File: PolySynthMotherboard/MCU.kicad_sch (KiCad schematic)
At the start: 45 parts, among them J201 SWD Header, J202 USB_C_Leceptacle_USB2.0, J203 MIDI_In, J204 MIDI_Thru, J205 MIDI_Out, J401 Micro_SD_Card_Det2, SW201 RST, SW202 BOOT, U201 STM32F411RETx, U202 74HC595, U203 74HC595, U204 4N35, U205 74HC04, Y201 16MHz, Y202 32.768kHZ

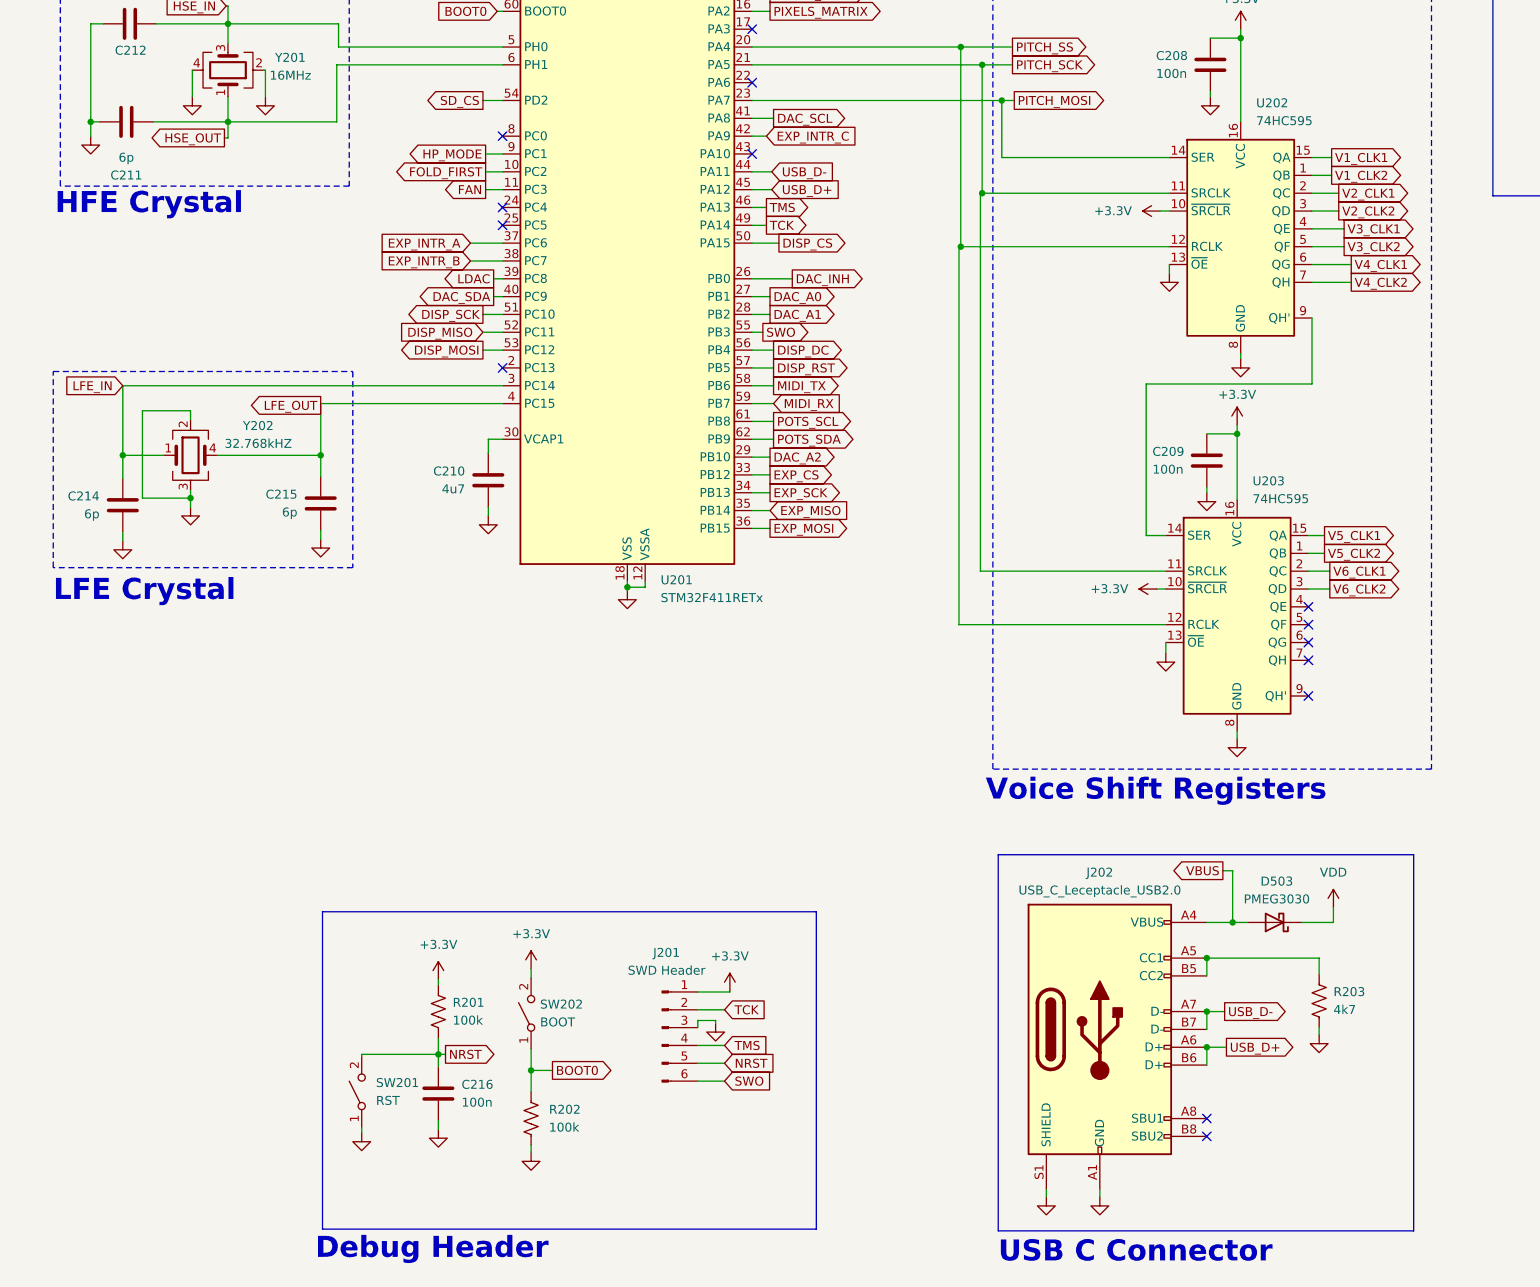
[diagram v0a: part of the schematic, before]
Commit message: motherboard rev1
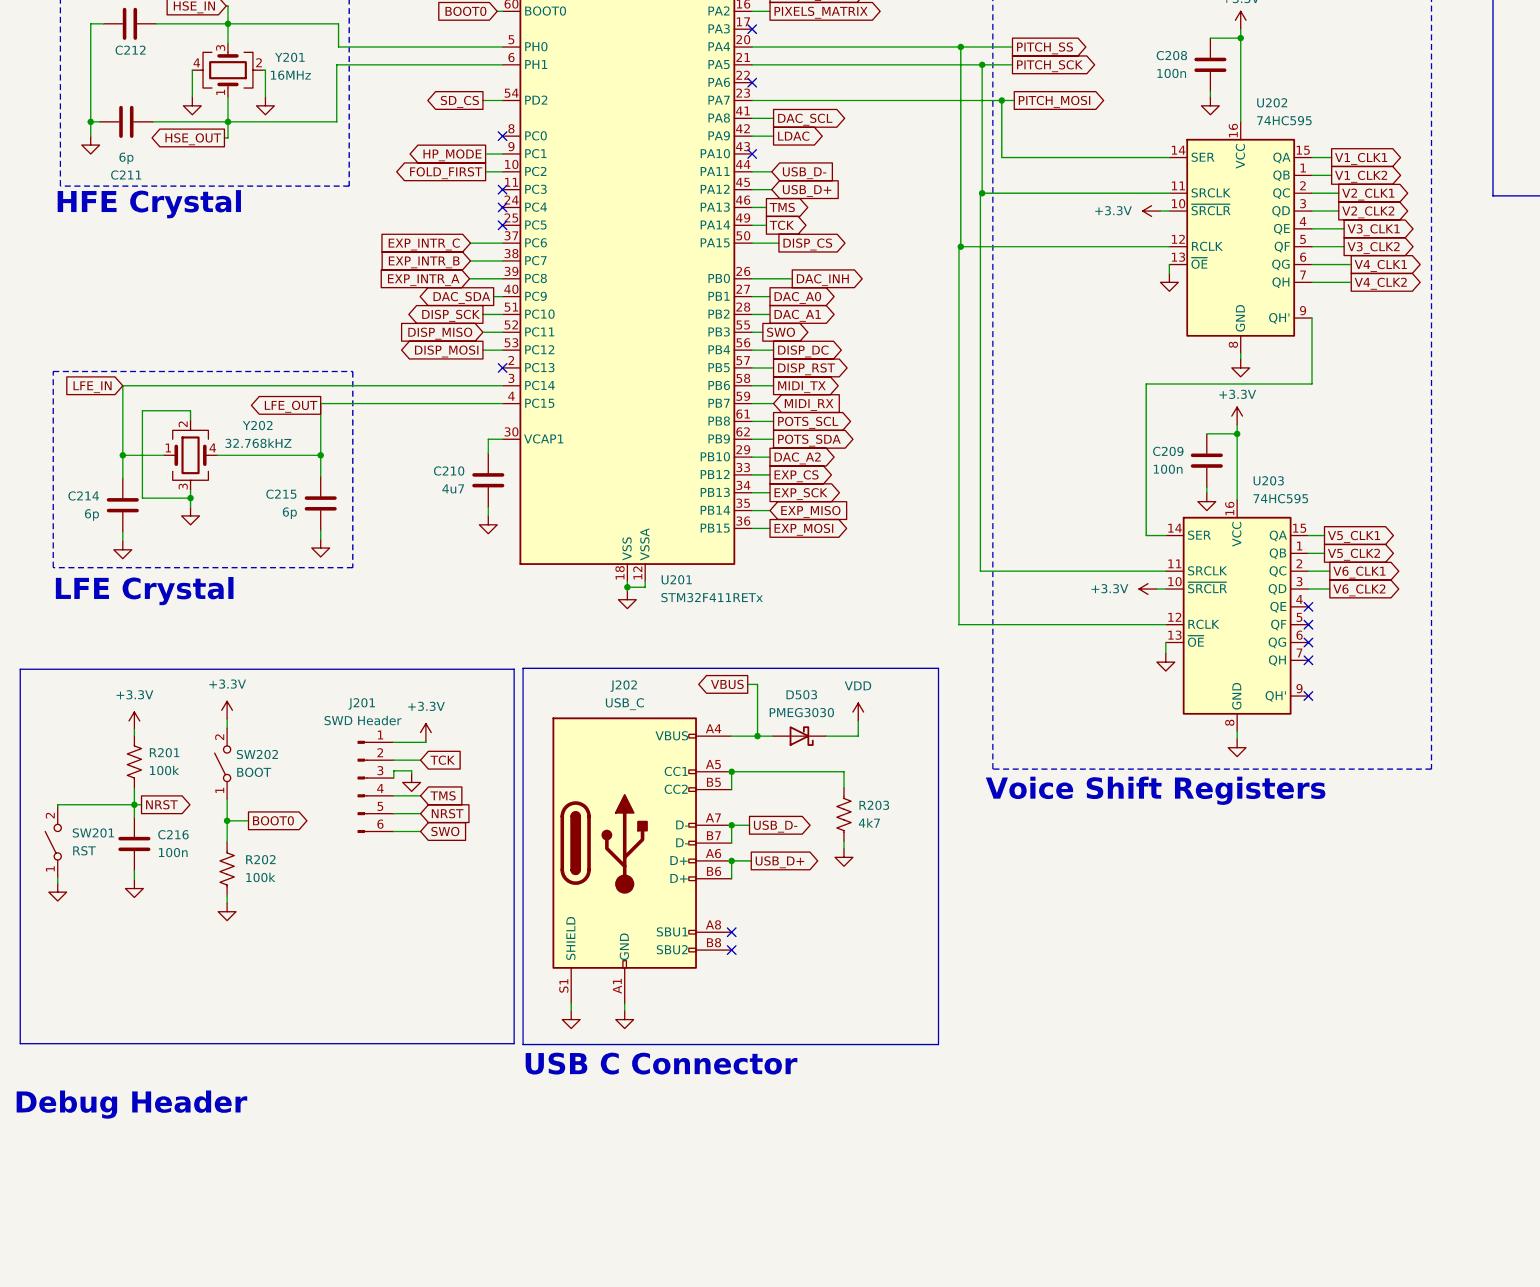
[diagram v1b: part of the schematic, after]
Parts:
- J202: value USB_C_Leceptacle_USB2.0 -> USB_C
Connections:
- net EXP_INTR_A: now also U201.39 (PC8); no longer U201.37 (PC6)
- net EXP_INTR_C: now also U201.37 (PC6); no longer U201.42 (PA9)
- net LDAC: now also U201.42 (PA9); no longer U201.39 (PC8)
- net FAN: no longer names the net of U201.11 (PC3)
- no-connect marks 23 -> 24
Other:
- moved on the sheet: C216, D503, J201, J202, R201, R202, R203, SW201, SW202
